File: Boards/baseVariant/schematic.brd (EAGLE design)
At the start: 93 x 70 mm, 99 parts, among them IC1 LM2596S, J1 AVR_SPI_PRG_6NS, U1 MAGJACK-POE, U2 MAGJACK-POE

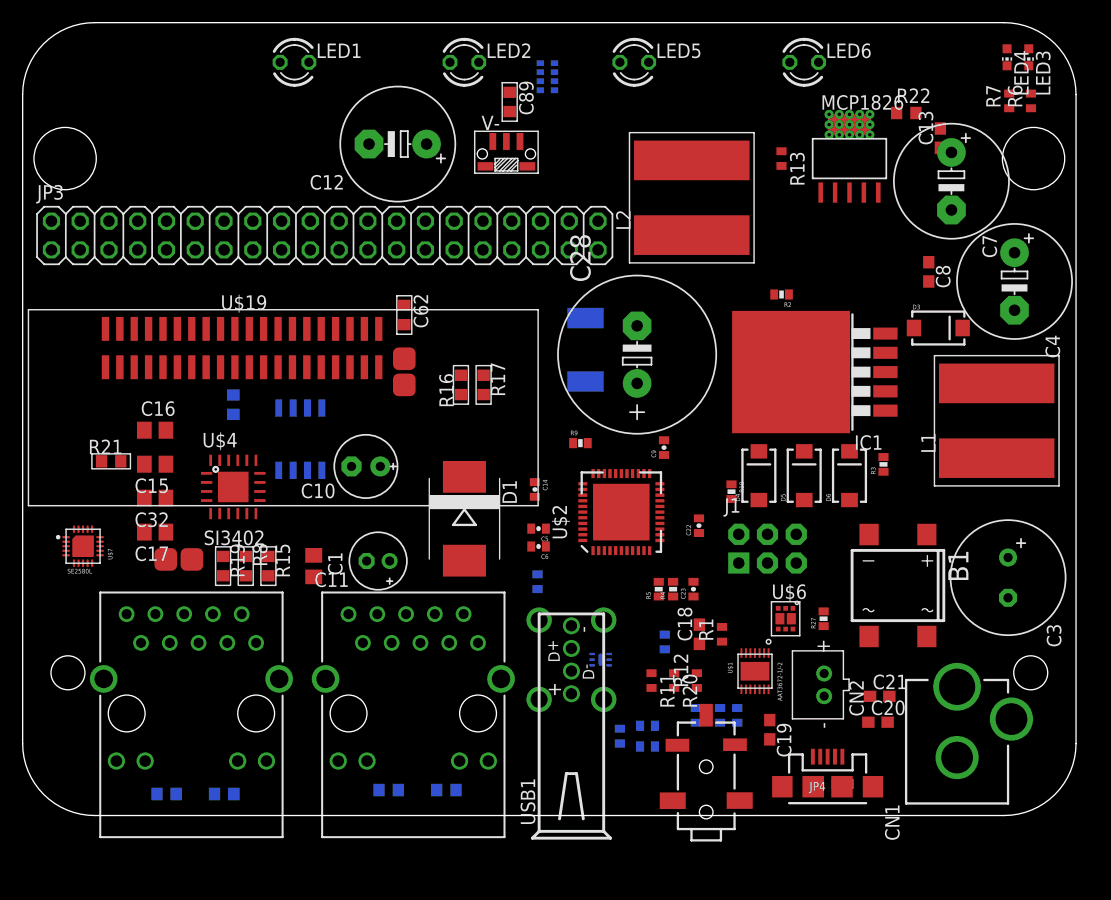
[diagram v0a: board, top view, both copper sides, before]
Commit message: normal Push.
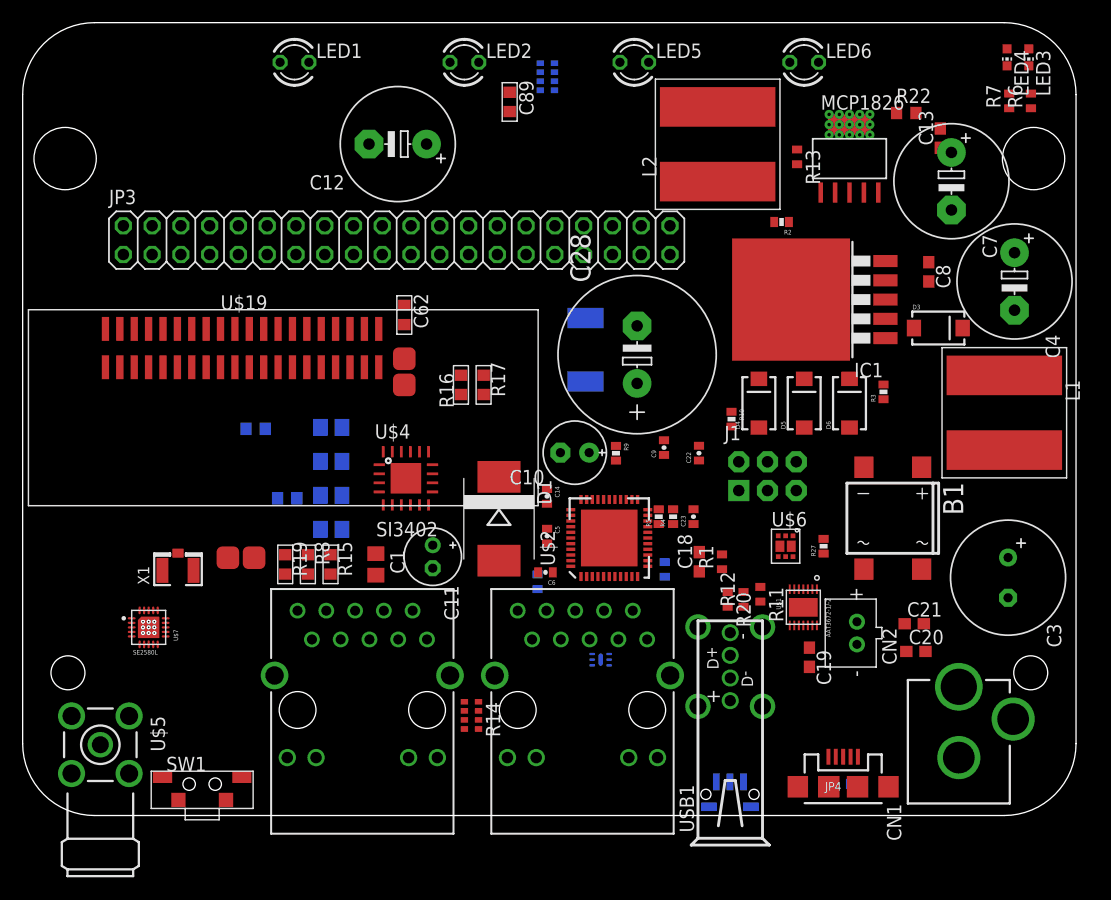
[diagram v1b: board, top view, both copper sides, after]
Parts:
- removed C2, C25: 1uF, SparkFun:0402-CAP
- removed JP1: (no value), SparkFun-Connectors:STEREOJACK2.5MM
- removed R23, R24, R25: 22, SparkFun:0402-RES
- removed R47, R48, R53, R54: 330R, BaseApp:R0603
- added SW1: (no value), BaseApp:TACTILE-2PIN-RTANGLE
- added X1: (no value), adafruit:U.FL
- R14: value 22 -> 330; device SparkFun:0402-RES -> SparkFun-Passives:0603-ARV
- R3: value (none) -> 1k
- R6, R7: value 57.6k -> 1.5k
- U$5: value MAX5556ESA+ -> RF-SMA; device schematic:SO-8 -> BaseApp:BU-SMA-H
- moved V- 59.9 mm to (62.4, 0.77), flipped to the bottom
- moved U$5 32.6 mm to (6.86, 6.25), flipped to the top, turned to 270 degrees
- moved R14 23.5 mm to (39.6, 8.84), flipped to the top
- moved C10 18.5 mm to (48.7, 32.0)
- moved C17 18.1 mm to (27.2, 34.3), flipped to the bottom, turned to 0 degrees
- moved C16 17.8 mm to (27.2, 25.3), flipped to the bottom, turned to 180 degrees
- moved R21 15.9 mm to (23.4, 28.0), flipped to the bottom, turned to 180 degrees
- moved C32 15.9 mm to (27.2, 31.3), flipped to the bottom, turned to 0 degrees
- moved C15 15.8 mm to (27.2, 28.3), flipped to the bottom, turned to 0 degrees
- moved U$4 15.3 mm to (33.8, 29.8)
- moved U2 15.1 mm to (30.0, 9.19)
- moved U1 14.9 mm to (49.4, 9.19)
- moved USB1 14.0 mm to (59.0, -2.61)
- moved R11 12.3 mm to (65.1, 19.5)
- moved U$7 9.21 mm to (11.1, 16.6)
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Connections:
- removed net N$1: U$7.P$16
- removed net N$14: C20.2, U$1.P$14
- removed net N$21: U$7.P$8
- removed net N$27: R14.2, R23.2
- removed net N$35: R24.2, R25.2
- removed net N$49: C2.2, JP1.4, R14.1
- removed net N$51: C25.2, JP1.1, R24.1
- removed net N$53: U$7.P$15
- removed net N$55: U$7.P$2
- removed net N$56: U$7.P$3
- removed net N$57: U$7.P$4
- removed net OUTL: C25.1, R25.1, U$5.8
- removed net OUTR: C2.1, R23.1, U$5.5
- new net RF2_OUT: U$5.1, U$7.P$15
- new net VLITHIUM: C20.2, MCP1826.2, U$1.P$14
- net ETH0_GRN+: now also R14.4; no longer R54.2
- net GND: now also R14.2, R14.3, U$5.2, U$5.3, U$5.4, U$5.5, U$7.P$2, U$7.P$4, X1.1, X1.2; no longer JP1.5, R47.2, R53.2, U$5.6
- net I2S_CK: no longer U$5.2
- net I2S_MCK: no longer U$5.4
- net I2S_SD: no longer U$5.1
- net I2S_WS: no longer U$5.3
- net JUMPSTART: now also SW1.2
- net N$24: now also R14.6; no longer R53.1
- net N$25: now also R14.1; no longer R48.1
- net N$31: now also R14.7; no longer R47.1
- net N$54: now also X1.3
- net N$95: now also R14.5; no longer R54.1
- net VCC: no longer MCP1826.2, U$5.7
- net VDD: now also R14.8, SW1.1, U$7.P$16, U$7.P$3, U$7.P$8; no longer R48.2
